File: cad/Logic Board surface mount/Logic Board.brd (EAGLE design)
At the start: 43 x 46 mm, 23 parts, among them Q1 8/16/20MHz, U1 ATMEGA328, U2 MIC5205

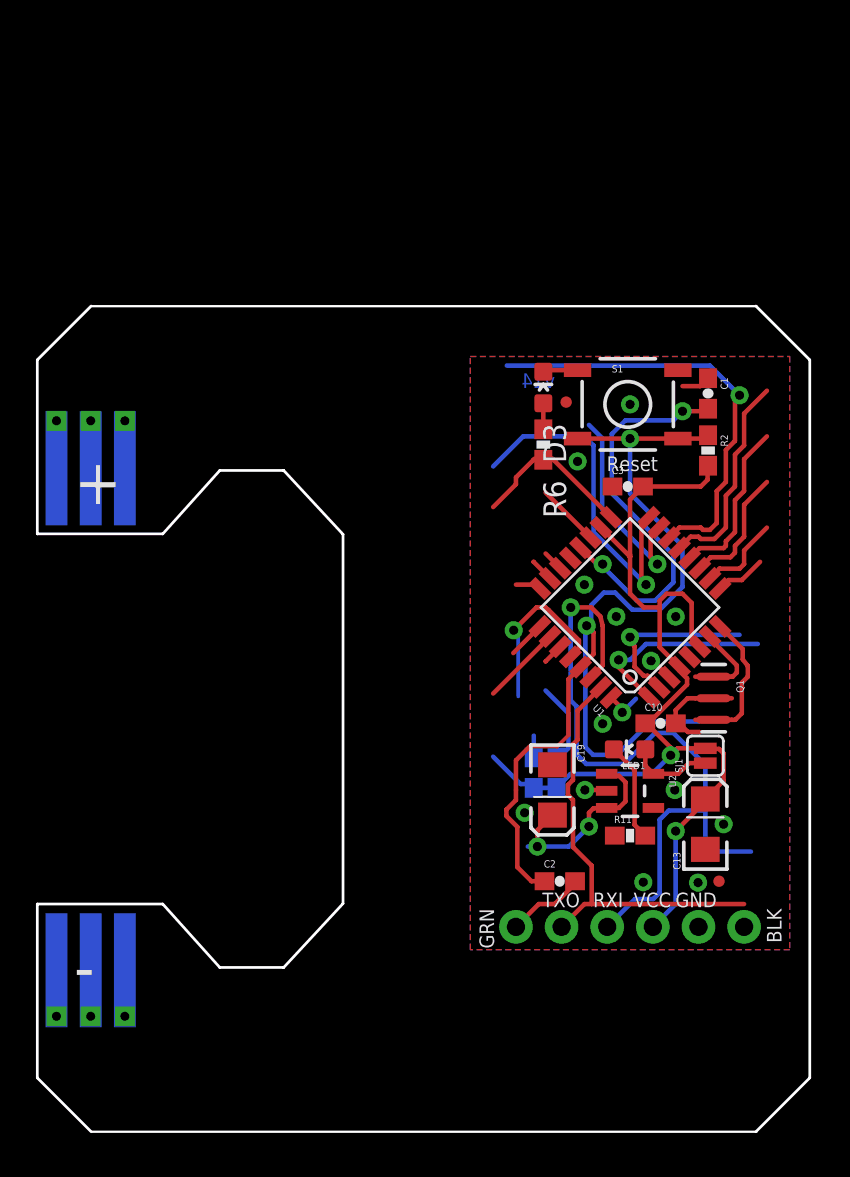
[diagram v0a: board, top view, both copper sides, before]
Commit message: Updated board
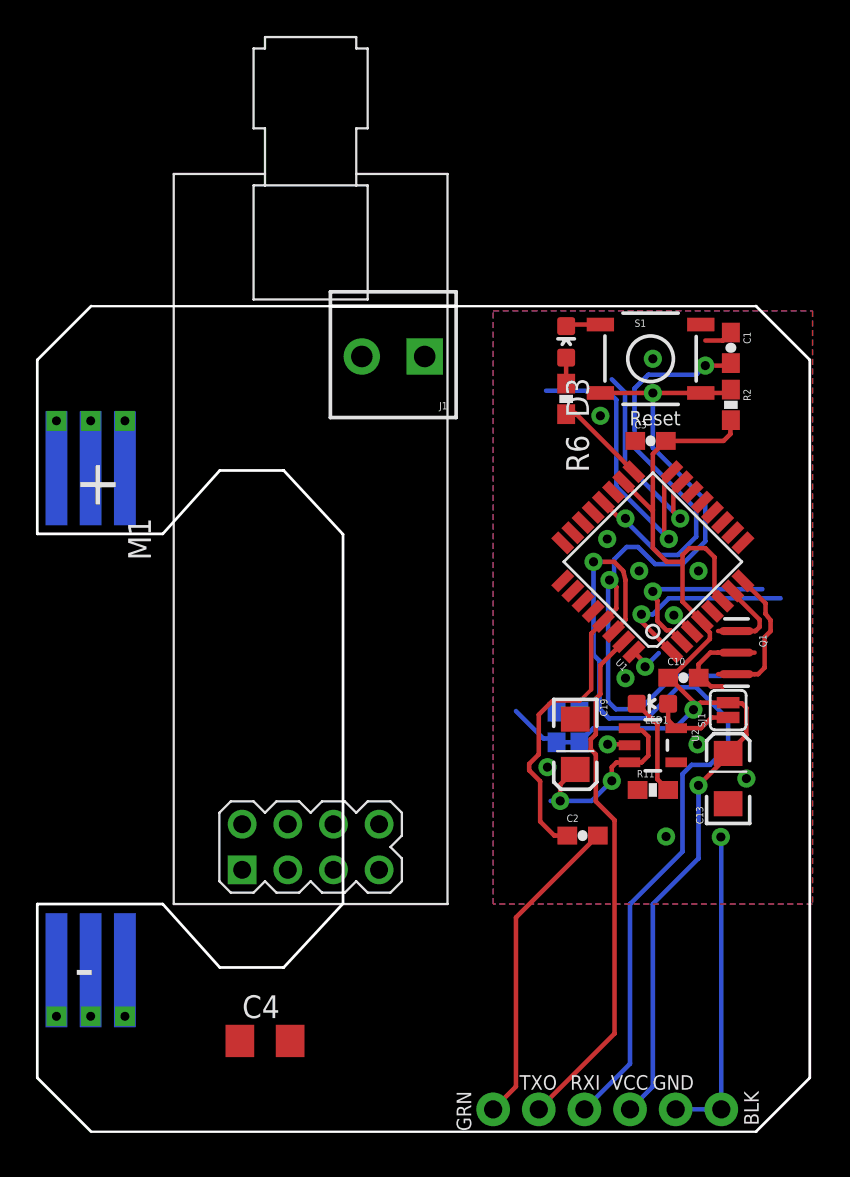
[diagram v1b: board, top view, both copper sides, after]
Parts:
- removed JP5, JP8: FIDUCIALUFIDUCIAL, SparkFun:MICRO-FIDUCIAL
- added C4: 10uF, rcl:C1206
- added J1: (no value), SparkFun-Connectors:SCREWTERMINAL-3.5MM-2
- added M1: WIRELESS-NRF24L01-PA-EXT, diy-modules:WIRELESS-NRD24L01-PA-EXT
- moved JP1 10.2 mm to (25.4, 1.27)
- moved SJ1 2.84 mm to (38.5, 23.5)
- moved C2 2.84 mm to (30.4, 16.5)
- moved C1 2.84 mm to (38.6, 43.7)
- moved C13 2.84 mm to (38.5, 19.7)
- moved LED1 2.84 mm to (34.3, 23.9)
- moved Q1 2.84 mm to (38.9, 26.7)
- moved R1 2.84 mm to (30.2, 22.6)
- moved R2 2.84 mm to (38.6, 40.5)
- moved U2 2.84 mm to (34.3, 21.5)
- moved C19 2.84 mm to (30.0, 21.6)
- moved D3 2.84 mm to (29.5, 44.0)
- moved R3 2.84 mm to (28.9, 22.6)
- moved R6 2.84 mm to (29.5, 40.8)
- moved C10 2.84 mm to (36.0, 25.3)
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- renumbered B1 to B2
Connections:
- new net BOUT: B2.B+, B2.B+@2
- new net GOUT: B2.G+, B2.G+@1
- new net N$10: B2.B-, B2.B-@1
- new net N$5: B2.R-, B2.R-@1
- new net N$9: B2.G-, B2.G-@1
- new net ROUT: B2.R+, B2.R+@1
- net D10: now also M1.4
- net D2: now also M1.8
- net D9: now also M1.3
- net GND: now also C4.2, J1.1, M1.1
- net MISO: now also M1.7
- net MOSI: now also M1.6
- net RAW: now also J1.2
- net SCK: now also M1.5
- net VCC: now also C4.1, M1.2
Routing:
- net D10: track 24.4 -> 0.00 mm, vias 1 -> 0
- net GND: track 9.36 -> 27.1 mm
- net VCC: track 56.8 -> 70.5 mm
- net DTR: track 4.42 -> 17.8 mm
- net D9: track 11.7 -> 0.00 mm
- net A5: track 11.0 -> 0.00 mm, vias 1 -> 0
- net D8: track 9.34 -> 0.00 mm
- net RXI: track 40.2 -> 48.3 mm
- net D7: track 6.99 -> 0.00 mm
- net A4: track 6.04 -> 0.00 mm
- net TXO: track 24.1 -> 29.1 mm
- net D6: track 4.79 -> 0.00 mm
- net A3: track 4.48 -> 0.00 mm
- net SCK: track 9.42 -> 5.20 mm
- net A6: track 3.55 -> 0.00 mm
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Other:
- board text removed: "v14"

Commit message: More board layout changes
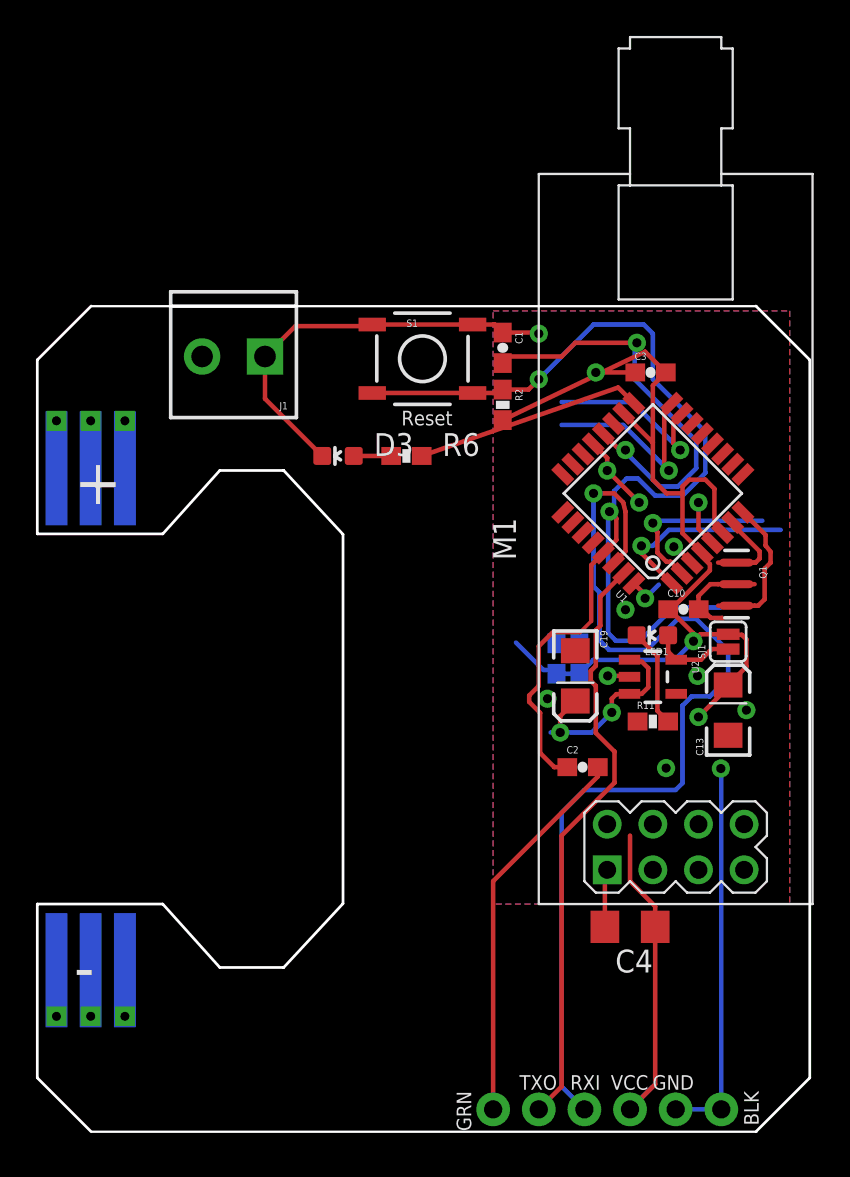
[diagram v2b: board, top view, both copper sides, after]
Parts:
- moved C4 21.3 mm to (33.0, 11.4), turned to 180 degrees
- moved M1 20.3 mm to (35.6, 33.0)
- moved D3 14.2 mm to (16.8, 37.6), turned to 90 degrees
- moved C1 12.7 mm to (25.9, 43.7)
- moved R2 12.7 mm to (25.9, 40.5)
- moved S1 12.7 mm to (21.5, 43.1)
- moved R6 9.44 mm to (20.6, 37.6), turned to 180 degrees
- moved J1 8.89 mm to (12.7, 43.2)
- moved C13 3.81 mm to (38.5, 23.5)
- moved Q1 3.81 mm to (38.9, 30.5)
- moved R1 3.81 mm to (30.2, 26.4)
- moved R3 3.81 mm to (28.9, 26.4)
- moved U1 3.81 mm to (34.3, 35.6)
- moved C10 3.81 mm to (36.0, 29.1)
- moved C19 3.81 mm to (30.0, 25.4)
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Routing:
- net GND: track 27.1 -> 63.2 mm
- net RESET: track 57.0 -> 66.5 mm
- net RXI: track 48.3 -> 56.1 mm
- net SCK: track 5.20 -> 12.8 mm
- net MISO: track 17.1 -> 11.0 mm
- net VCC: track 70.5 -> 75.0 mm
- net TXO: track 29.1 -> 32.9 mm
- net DTR: track 17.8 -> 21.6 mm
- net MOSI: track 11.7 -> 10.1 mm
- net AREF: track 22.8 -> 23.6 mm
- net N$7: track 1.45 -> 2.08 mm
- added copper zone on layer 1, net VCC
- removed copper zone on layer 1, net GND
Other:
- board text added: "TODO: - Replace all headers with SMT - Replace 0603 components with 1206"
